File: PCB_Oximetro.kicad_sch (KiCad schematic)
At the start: 14 parts, among them J1 Conn_01x05, J2 Conn_01x08, J3 USB_B_Micro, SW1 SW_Push, U3 LM1117MP-3.3, U5 ESP32-DEVKIT-V1

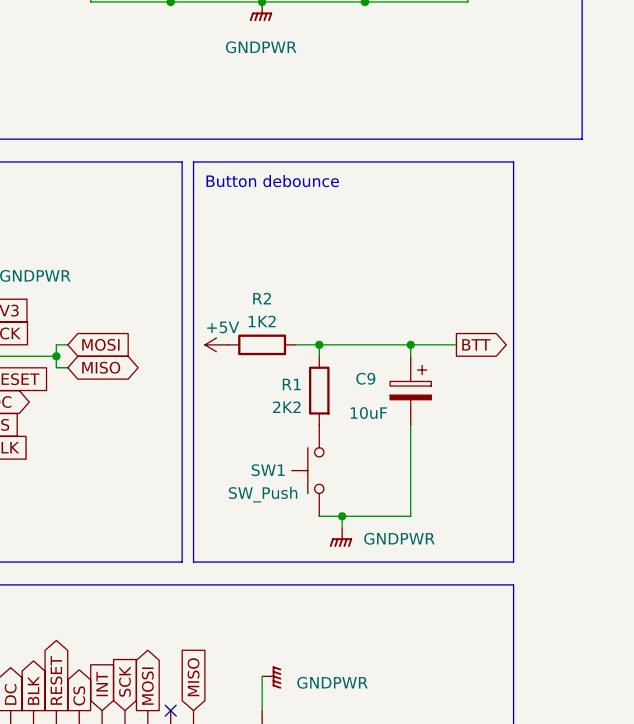
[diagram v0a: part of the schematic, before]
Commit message: BTT Update
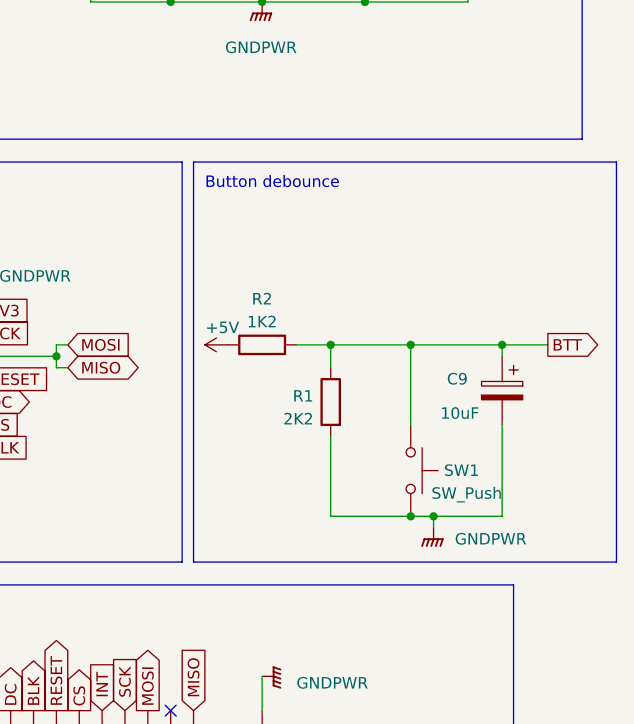
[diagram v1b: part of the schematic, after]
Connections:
- net BTT: now also SW1.2
- net GNDPWR: now also R1.2
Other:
- moved on the sheet: C9, R1, SW1
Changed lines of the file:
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@@
     (date "2023-09-05")
   )
-  (junction (at 95.25 95.25) (diameter 0) (color 0 0 0 0)
+  (junction (at 105.41 95.25) (diameter 0) (color 0 0 0 0)
+  )
+  (junction (at 93.98 76.2) (diameter 0) (color 0 0 0 0)
   )
   (junction (at 97.79 29.21) (diameter 0) (color 0 0 0 0)
@@
   (junction (at 63.5 77.47) (diameter 0) (color 0 0 0 0)
   )
+  (junction (at 113.03 76.2) (diameter 0) (color 0 0 0 0)
+  )
   (junction (at 102.87 76.2) (diameter 0) (color 0 0 0 0)
   )
-  (junction (at 92.71 76.2) (diameter 0) (color 0 0 0 0)
-  )
   (junction (at 109.22 29.21) (diameter 0) (color 0 0 0 0)
   )
@@
   )
   (junction (at 86.36 38.1) (diameter 0) (color 0 0 0 0)
+  )
+  (junction (at 102.87 95.25) (diameter 0) (color 0 0 0 0)
   )
   (no_connect (at 76.2 147.32))
@@
     (stroke (width 0) (type default))
   )
-  (wire (pts (xy 92.71 77.47) (xy 92.71 76.2))
+  (wire (pts (xy 93.98 86.36) (xy 93.98 95.25))
+    (stroke (width 0) (type default))
+  )
+  (wire (pts (xy 102.87 76.2) (xy 102.87 85.09))
     (stroke (width 0) (type default))
   )
@@
     (stroke (width 0) (type default))
   )
-  (wire (pts (xy 95.25 95.25) (xy 92.71 95.25))
-    (stroke (width 0) (type default))
-  )
-  (wire (pts (xy 102.87 76.2) (xy 107.95 76.2))
-    (stroke (width 0) (type default))
-  )
-  (wire (pts (xy 102.87 85.09) (xy 102.87 95.25))
+  (wire (pts (xy 105.41 95.25) (xy 102.87 95.25))
+    (stroke (width 0) (type default))
+  )
+  (wire (pts (xy 93.98 76.2) (xy 90.17 76.2))
+    (stroke (width 0) (type default))
+  )
+  (wire (pts (xy 113.03 76.2) (xy 118.11 76.2))
+    (stroke (width 0) (type default))
+  )
+  (wire (pts (xy 113.03 85.09) (xy 113.03 95.25))
     (stroke (width 0) (type default))
   )
@@
     (stroke (width 0) (type default))
   )
+  (wire (pts (xy 93.98 78.74) (xy 93.98 76.2))
+    (stroke (width 0) (type default))
+  )
   (wire (pts (xy 21.59 44.45) (xy 22.86 44.45))
     (stroke (width 0) (type default))
@@
     (stroke (width 0) (type default))
   )
-  (wire (pts (xy 95.25 95.25) (xy 95.25 96.52))
+  (wire (pts (xy 105.41 95.25) (xy 105.41 96.52))
     (stroke (width 0) (type default))
   )
@@
     (stroke (width 0) (type default))
   )
-  (wire (pts (xy 102.87 77.47) (xy 102.87 76.2))
+  (wire (pts (xy 113.03 77.47) (xy 113.03 76.2))
     (stroke (width 0) (type default))
   )
@@
     (stroke (width 0) (type default))
   )
-  (wire (pts (xy 102.87 95.25) (xy 95.25 95.25))
+  (wire (pts (xy 113.03 95.25) (xy 105.41 95.25))
     (stroke (width 0) (type default))
   )
@@
     (stroke (width 0) (type default))
   )
+  (wire (pts (xy 93.98 95.25) (xy 102.87 95.25))
+    (stroke (width 0) (type default))
+  )
   (wire (pts (xy 76.2 29.21) (xy 78.74 29.21))
     (stroke (width 0) (type default))
@@
     (stroke (width 0) (type default))
   )
-  (wire (pts (xy 102.87 76.2) (xy 92.71 76.2))
+  (wire (pts (xy 113.03 76.2) (xy 102.87 76.2))
     (stroke (width 0) (type default))
   )
@@
     (stroke (width 0) (type default))
   )
-  (wire (pts (xy 92.71 76.2) (xy 90.17 76.2))
+  (wire (pts (xy 93.98 76.2) (xy 102.87 76.2))
     (stroke (width 0) (type default))
   )
@@
     (fill (type none))
   )
-  (rectangle (start 78.74 55.88) (end 114.3 100.33)
+  (rectangle (start 78.74 55.88) (end 125.73 100.33)
     (stroke (width 0) (type default))
     (fill (type none))
@@
     )
   )
-  (global_label "BTT" (shape output) (at 107.95 76.2 0) (fields_autoplaced)
-    (effects (font (size 1.27 1.27)) (justify left))
-    (property "Intersheetrefs" "${INTERSHEET_REFS}" (at 114.061 76.2 0)
+  (global_label "BTT" (shape output) (at 118.11 76.2 0) (fields_autoplaced)
+    (effects (font (size 1.27 1.27)) (justify left))
+    (property "Intersheetrefs" "${INTERSHEET_REFS}" (at 124.221 76.2 0)
       (effects (font (size 1.27 1.27)) (justify left) hide)
     )
@@
     )
   )
-  (symbol (lib_id "Device:R") (at 92.71 81.28 0) (mirror y) (unit 1)
-    (in_bom yes) (on_board yes) (dnp no)
-    (property "Reference" "R1" (at 90.805 80.645 0)
-      (effects (font (size 1.27 1.27)) (justify left))
-    )
-    (property "Value" "2K2" (at 90.805 83.185 0)
-      (effects (font (size 1.27 1.27)) (justify left))
-    )
-    (property "Footprint" "Resistor_SMD:R_1206_3216Metric" (at 94.488 81.28 90)
-      (effects (font (size 1.27 1.27)) hide)
-    )
-    (property "Datasheet" "~" (at 92.71 81.28 0)
+  (symbol (lib_id "Device:R") (at 93.98 82.55 0) (mirror y) (unit 1)
+    (in_bom yes) (on_board yes) (dnp no)
+    (property "Reference" "R1" (at 92.075 81.915 0)
+      (effects (font (size 1.27 1.27)) (justify left))
+    )
+    (property "Value" "2K2" (at 92.075 84.455 0)
+      (effects (font (size 1.27 1.27)) (justify left))
+    )
+    (property "Footprint" "Resistor_SMD:R_1206_3216Metric" (at 95.758 82.55 90)
+      (effects (font (size 1.27 1.27)) hide)
+    )
+    (property "Datasheet" "~" (at 93.98 82.55 0)
       (effects (font (size 1.27 1.27)) hide)
     )
@@
     )
   )
-  (symbol (lib_id "power:GNDPWR") (at 95.25 96.52 0) (unit 1)
-    (in_bom yes) (on_board yes) (dnp no)
-    (property "Reference" "#PWR05" (at 95.25 101.6 0)
-      (effects (font (size 1.27 1.27)) hide)
-    )
-    (property "Value" "GNDPWR" (at 101.6 97.79 0)
-      (effects (font (size 1.27 1.27)))
-    )
-    (property "Footprint" "" (at 95.25 97.79 0)
-      (effects (font (size 1.27 1.27)) hide)
-    )
-    (property "Datasheet" "" (at 95.25 97.79 0)
+  (symbol (lib_id "power:GNDPWR") (at 105.41 96.52 0) (unit 1)
+    (in_bom yes) (on_board yes) (dnp no)
+    (property "Reference" "#PWR05" (at 105.41 101.6 0)
+      (effects (font (size 1.27 1.27)) hide)
+    )
+    (property "Value" "GNDPWR" (at 111.76 97.79 0)
+      (effects (font (size 1.27 1.27)))
+    )
+    (property "Footprint" "" (at 105.41 97.79 0)
+      (effects (font (size 1.27 1.27)) hide)
+    )
+    (property "Datasheet" "" (at 105.41 97.79 0)
       (effects (font (size 1.27 1.27)) hide)
     )
@@
     )
   )
-  (symbol (lib_id "Switch:SW_Push") (at 92.71 90.17 90) (unit 1)
-    (in_bom yes) (on_board yes) (dnp no)
-    (property "Reference" "SW1" (at 85.09 90.17 90)
+  (symbol (lib_id "Switch:SW_Push") (at 102.87 90.17 270) (mirror x) (unit 1)
+    (in_bom yes) (on_board yes) (dnp no)
+    (property "Reference" "SW1" (at 110.49 90.17 90)
       (effects (font (size 1.27 1.27)) (justify right))
     )
-    (property "Value" "SW_Push" (at 82.55 92.71 90)
+    (property "Value" "SW_Push" (at 113.03 92.71 90)
       (effects (font (size 1.27 1.27)) (justify right))
     )
-    (property "Footprint" "Button_Switch_THT:SW_Tactile_SPST_Angled_PTS645Vx58-2LFS" (at 87.63 90.17 0)
-      (effects (font (size 1.27 1.27)) hide)
-    )
-    (property "Datasheet" "~" (at 87.63 90.17 0)
+    (property "Footprint" "Button_Switch_THT:SW_Tactile_SPST_Angled_PTS645Vx58-2LFS" (at 107.95 90.17 0)
+      (effects (font (size 1.27 1.27)) hide)
+    )
+    (property "Datasheet" "~" (at 107.95 90.17 0)
       (effects (font (size 1.27 1.27)) hide)
     )
@@
     )
   )
-  (symbol (lib_id "Device:C_Polarized") (at 102.87 81.28 0) (mirror y) (unit 1)
-    (in_bom yes) (on_board yes) (dnp no)
-    (property "Reference" "C9" (at 99.06 80.01 0)
-      (effects (font (size 1.27 1.27)) (justify left))
-    )
-    (property "Value" "10uF" (at 100.33 83.82 0)
-      (effects (font (size 1.27 1.27)) (justify left))
-    )
-    (property "Footprint" "Capacitor_THT:CP_Radial_D5.0mm_P2.50mm" (at 101.9048 85.09 0)
-      (effects (font (size 1.27 1.27)) hide)
-    )
-    (property "Datasheet" "~" (at 102.87 81.28 0)
-      (effects (font (size 1.27 1.27)) hide)
-    )
+  (symbol (lib_id "Device:C_Polarized") (at 113.03 81.28 0) (mirror y) (unit 1)
+    (in_bom yes) (on_board yes) (dnp no)
+    (property "Reference" "C9" (at 109.22 80.01 0)
+      (effects (font (size 1.27 1.27)) (justify left))
+    )
+    (property "Value" "10uF" (at 110.49 83.82 0)
+      (effects (font (size 1.27 1.27)) (justify left))
+    )
+    (property "Footprint" "Capacitor_THT:CP_Radial_D5.0mm_P2.50mm" (at 112.0648 85.09 0)
+      (effects (font (size 1.27 1.27)) hide)
+    )
+    (property "Datasheet" "~" (at 113.03 81.28 0)
+      (effects (font (size 1.27 1.27)) hide)
+    )
